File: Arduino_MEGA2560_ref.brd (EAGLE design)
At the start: 101.6 x 53.3 mm, 72 parts, among them IC1 MC33269ST-5.0T3, IC2 MC33269D-5.0, IC3 ATMEGA2560-16AU, IC4 ATMEGA8U2-MU, IC5 LM358D, IC6 LP2985-33DBVR, Q1 16MHz, Q2 16MHz, T2 FDN340P, X1 DC21MMX, Y1 16MHz, Y2 16MHz

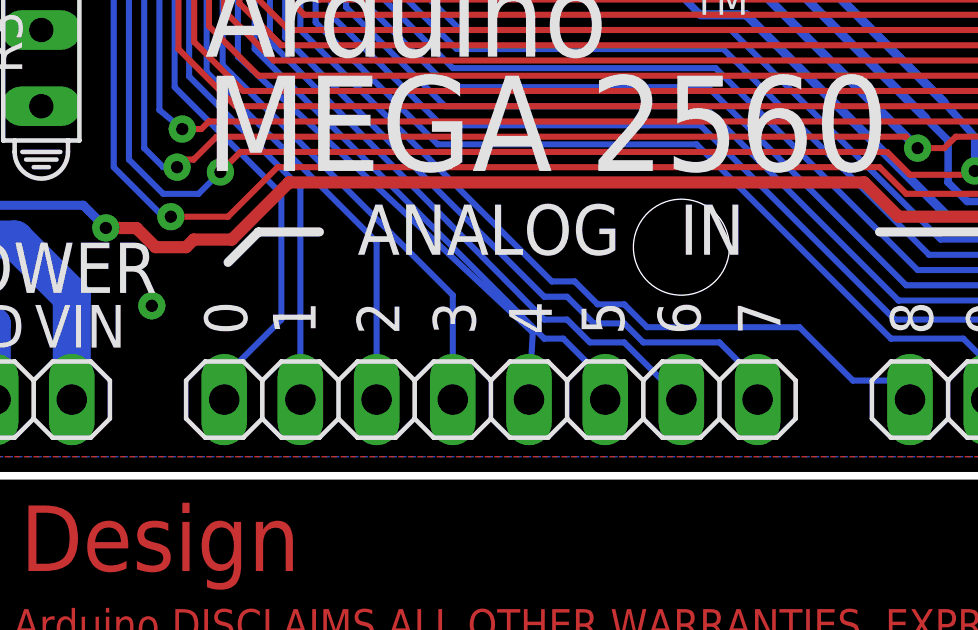
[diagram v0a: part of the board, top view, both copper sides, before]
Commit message: master changes
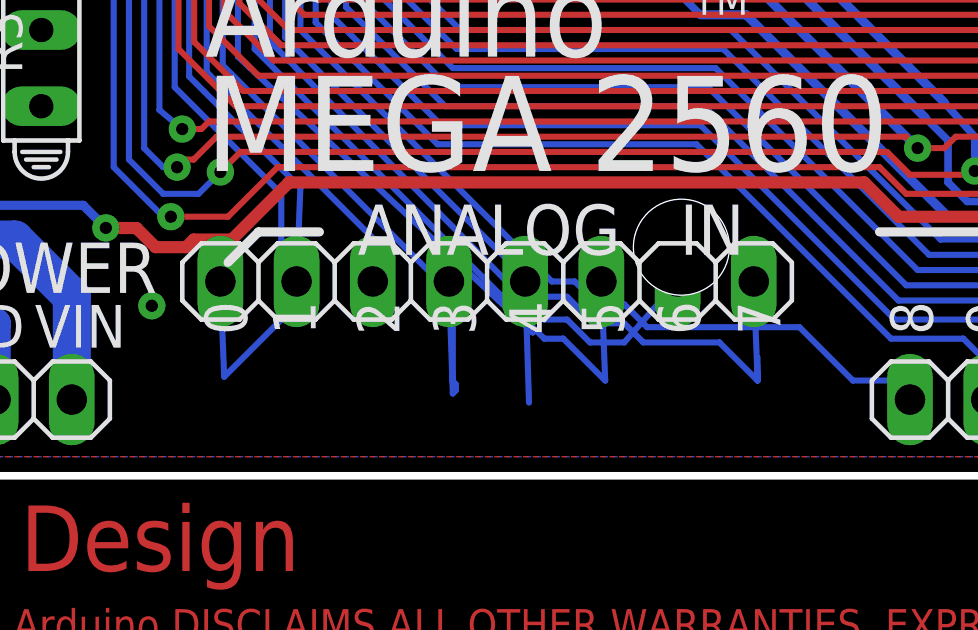
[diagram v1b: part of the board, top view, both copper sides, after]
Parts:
- moved ADCL 3.94 mm to (59.6, 6.48)
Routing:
- net ADC1: track 44.4 -> 40.5 mm
- net ADC2: track 46.9 -> 42.9 mm
- net ADC3: track 49.7 -> 53.3 mm
- net ADC4: track 52.9 -> 56.3 mm
- net ADC7: track 58.1 -> 60.8 mm
- net ADC5: track 55.9 -> 58.5 mm
- net ADC0: track 43.0 -> 45.4 mm
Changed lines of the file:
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@@
 <attribute name="VALUE" x="13.716" y="16.256" size="1.27" layer="27" rot="R90"/>
 </element>
-<element name="ADCL" library="pinhead" package="1X08" value="" x="59.69" y="2.54" smashed="yes">
-<attribute name="NAME" x="57.6326" y="4.7498" size="1.27" layer="49" ratio="10"/>
-<attribute name="VALUE" x="49.53" y="-0.635" size="1.27" layer="27"/>
+<element name="ADCL" library="pinhead" package="1X08" value="" x="59.563" y="6.477" smashed="yes">
+<attribute name="NAME" x="57.5056" y="8.6868" size="1.27" layer="49" ratio="10"/>
+<attribute name="VALUE" x="49.403" y="3.302" size="1.27" layer="27"/>
 </element>
 <element name="COMMUNICATION" library="pinhead" package="1X08" value="" x="77.47" y="50.8" smashed="yes" rot="R180">
@@
 <wire x1="52.705" y1="5.207" x2="52.705" y2="9.398" width="0.2032" layer="16"/>
 <wire x1="50.8" y1="3.302" x2="52.705" y2="5.207" width="0.2032" layer="16"/>
-<wire x1="50.8" y1="2.54" x2="50.8" y2="3.302" width="0.2032" layer="16"/>
+<wire x1="50.673" y1="6.477" x2="50.8" y2="3.302" width="0.2032" layer="16"/>
 <wire x1="46.3" y1="37.52" x2="46.3" y2="36.3464" width="0.2032" layer="1"/>
 <wire x1="46.228" y1="25.273" x2="46.228" y2="37.592" width="0.2032" layer="16"/>
@@
 <contactref element="ADCL" pad="3"/>
 <contactref element="IC3" pad="95"/>
-<wire x1="55.88" y1="2.54" x2="55.88" y2="7.7978" width="0.2032" layer="16"/>
+<wire x1="55.753" y1="6.477" x2="55.88" y2="7.7978" width="0.2032" layer="16"/>
 <wire x1="47.371" y1="36.576" x2="47.3" y2="36.505" width="0.2032" layer="1"/>
 <wire x1="47.2694" y1="36.6776" x2="47.371" y2="36.576" width="0.2032" layer="1"/>
@@
 <wire x1="49.6316" y1="13.3096" x2="49.6316" y2="22.5552" width="0.2032" layer="16"/>
 <wire x1="53.34" y1="9.6012" x2="49.6316" y2="13.3096" width="0.2032" layer="16"/>
-<wire x1="53.34" y1="2.54" x2="53.34" y2="9.6012" width="0.2032" layer="16"/>
+<wire x1="53.213" y1="6.477" x2="53.34" y2="9.6012" width="0.2032" layer="16"/>
 <wire x1="46.8" y1="37.655" x2="46.8" y2="36.3464" width="0.2032" layer="1"/>
 <wire x1="46.482" y1="37.973" x2="46.8" y2="37.655" width="0.2032" layer="1"/>
@@
 <wire x1="58.42" y1="3.1496" x2="58.42" y2="6.0198" width="0.2032" layer="16"/>
 <wire x1="58.5216" y1="3.048" x2="58.42" y2="3.1496" width="0.2032" layer="16"/>
-<wire x1="58.42" y1="2.54" x2="58.42" y2="2.7432" width="0.2032" layer="16"/>
+<wire x1="58.293" y1="6.477" x2="58.42" y2="2.7432" width="0.2032" layer="16"/>
 <wire x1="58.5216" y1="2.8448" x2="58.5216" y2="3.048" width="0.2032" layer="16"/>
 <wire x1="58.42" y1="2.7432" x2="58.5216" y2="2.8448" width="0.2032" layer="16"/>
@@
 <wire x1="51.2572" y1="13.97" x2="51.2572" y2="23.0632" width="0.2032" layer="16"/>
 <wire x1="61.087" y1="4.7752" x2="51.2572" y2="13.97" width="0.2032" layer="16"/>
-<wire x1="60.96" y1="2.4384" x2="60.96" y2="2.54" width="0.2032" layer="16"/>
-<wire x1="60.96" y1="2.54" x2="61.087" y2="4.7752" width="0.2032" layer="16"/>
+<wire x1="60.96" y1="2.4384" x2="60.833" y2="6.477" width="0.2032" layer="16"/>
+<wire x1="60.833" y1="6.477" x2="61.087" y2="4.7752" width="0.2032" layer="16"/>
 <wire x1="48.3" y1="38.06" x2="48.3" y2="36.3464" width="0.2032" layer="1"/>
 <wire x1="48.006" y1="38.354" x2="48.3" y2="38.06" width="0.2032" layer="1"/>
@@
 <wire x1="62.103" y1="4.572" x2="61.468" y2="4.572" width="0.2032" layer="16"/>
 <wire x1="62.103" y1="4.572" x2="63.5" y2="3.175" width="0.2032" layer="16"/>
-<wire x1="63.5" y1="3.175" x2="63.5" y2="2.54" width="0.2032" layer="16"/>
+<wire x1="63.5" y1="3.175" x2="63.373" y2="6.477" width="0.2032" layer="16"/>
 <via x="49.657" y="43.561" extent="1-16" drill="0.4064" shape="octagon"/>
 </signal>
@@
 <wire x1="62.992" y1="4.445" x2="62.23" y2="5.207" width="0.2032" layer="16"/>
 <wire x1="62.992" y1="4.445" x2="64.135" y2="4.445" width="0.2032" layer="16"/>
-<wire x1="64.135" y1="4.445" x2="66.04" y2="2.54" width="0.2032" layer="16"/>
+<wire x1="64.135" y1="4.445" x2="65.913" y2="6.477" width="0.2032" layer="16"/>
 <via x="49.276" y="39.37" extent="1-16" drill="0.4064" shape="octagon"/>
 </signal>
@@
 <wire x1="52.832" y1="14.605" x2="52.832" y2="23.368" width="0.2032" layer="16"/>
 <wire x1="52.832" y1="14.605" x2="61.468" y2="5.969" width="0.2032" layer="16"/>
-<wire x1="68.58" y1="3.175" x2="68.58" y2="2.54" width="0.2032" layer="16"/>
+<wire x1="68.58" y1="3.175" x2="68.453" y2="6.477" width="0.2032" layer="16"/>
 <wire x1="68.58" y1="3.175" x2="68.58" y2="3.937" width="0.2032" layer="16"/>
 <wire x1="64.77" y1="4.445" x2="67.31" y2="4.445" width="0.2032" layer="16"/>

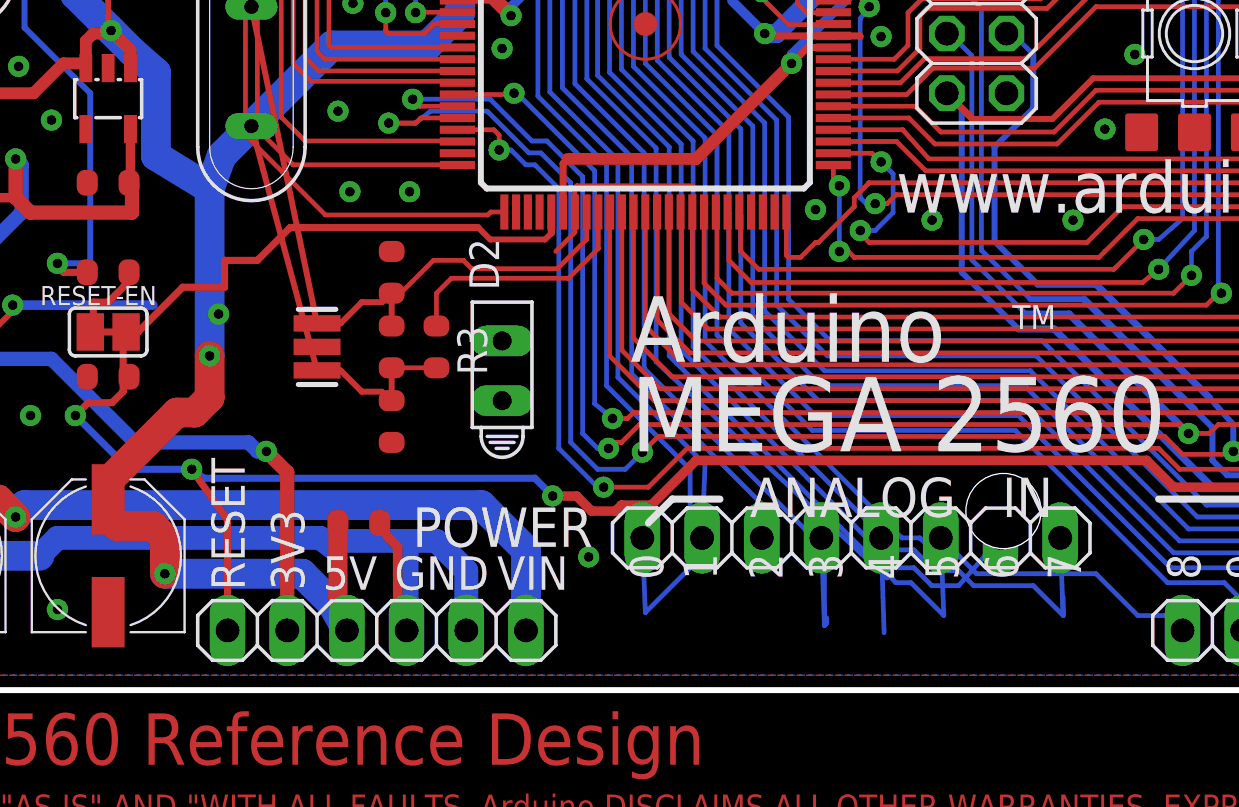
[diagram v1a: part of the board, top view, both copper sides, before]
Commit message: feature branch created with some changes
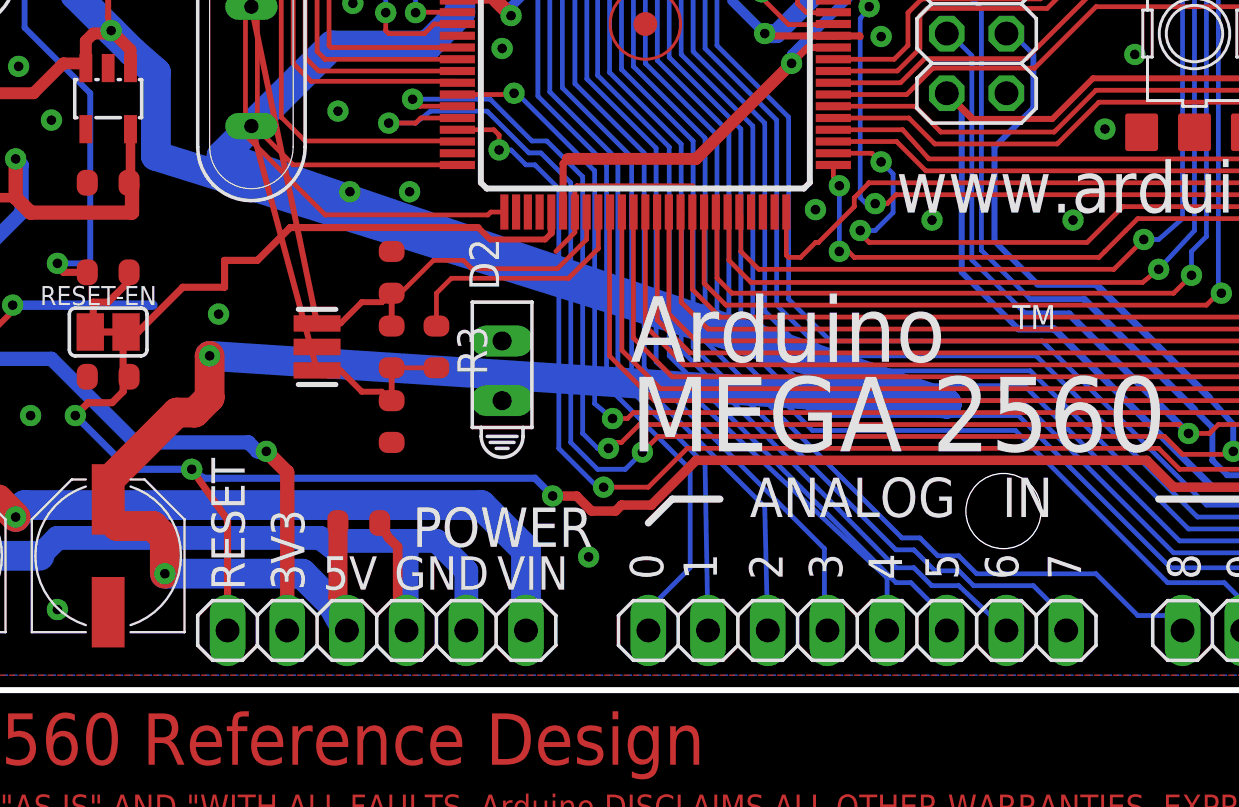
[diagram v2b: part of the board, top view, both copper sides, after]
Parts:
- moved ADCL 3.95 mm to (59.8, 2.54)
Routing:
- net +5V: track 291.7 -> 379.7 mm
- net ADC1: track 40.5 -> 44.4 mm
- net ADC2: track 42.9 -> 46.9 mm
- net ADC3: track 53.3 -> 49.8 mm
- net ADC4: track 56.3 -> 53.0 mm
- net ADC7: track 60.8 -> 58.1 mm
- net ADC5: track 58.5 -> 55.9 mm
- net ADC0: track 45.4 -> 43.0 mm
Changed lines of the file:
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@@
 <attribute name="VALUE" x="13.716" y="16.256" size="1.27" layer="27" rot="R90"/>
 </element>
-<element name="ADCL" library="pinhead" package="1X08" value="" x="59.563" y="6.477" smashed="yes">
-<attribute name="NAME" x="57.5056" y="8.6868" size="1.27" layer="49" ratio="10"/>
-<attribute name="VALUE" x="49.403" y="3.302" size="1.27" layer="27"/>
+<element name="ADCL" library="pinhead" package="1X08" value="" x="59.817" y="2.54" smashed="yes">
+<attribute name="NAME" x="57.7596" y="4.7498" size="1.27" layer="49" ratio="10"/>
+<attribute name="VALUE" x="49.657" y="-0.635" size="1.27" layer="27"/>
 </element>
 <element name="COMMUNICATION" library="pinhead" package="1X08" value="" x="77.47" y="50.8" smashed="yes" rot="R180">
@@
 <wire x1="18.796" y1="34.544" x2="18.038" y2="35.302" width="0.3048" layer="1"/>
 <wire x1="29.972" y1="22.733" x2="29.972" y2="26.289" width="1.27" layer="16"/>
-<wire x1="32.258" y1="21.336" x2="29.972" y2="22.733" width="1.27" layer="16"/>
-<wire x1="32.258" y1="14.224" x2="32.258" y2="21.336" width="1.27" layer="16"/>
+<wire x1="63.627" y1="12.192" x2="29.972" y2="22.733" width="1.27" layer="16"/>
+<wire x1="32.258" y1="14.224" x2="63.627" y2="12.192" width="1.27" layer="16"/>
 <wire x1="32.258" y1="14.224" x2="32.258" y2="14.986" width="0" layer="19" extent="1-16"/>
 <wire x1="37.465" y1="27.432" x2="41.529" y2="27.432" width="1.27" layer="16"/>
 <wire x1="32.766" y1="22.733" x2="37.465" y2="27.432" width="1.27" layer="16"/>
-<wire x1="32.258" y1="21.336" x2="32.766" y2="22.733" width="1.27" layer="16"/>
+<wire x1="63.627" y1="12.192" x2="32.766" y2="22.733" width="1.27" layer="16"/>
 <wire x1="29.972" y1="26.289" x2="28.956" y2="27.178" width="1.27" layer="16"/>
 <wire x1="28.956" y1="27.178" x2="28.067" y2="28.067" width="1.27" layer="16"/>
@@
 <wire x1="52.705" y1="5.207" x2="52.705" y2="9.398" width="0.2032" layer="16"/>
 <wire x1="50.8" y1="3.302" x2="52.705" y2="5.207" width="0.2032" layer="16"/>
-<wire x1="50.673" y1="6.477" x2="50.8" y2="3.302" width="0.2032" layer="16"/>
+<wire x1="50.927" y1="2.54" x2="50.8" y2="3.302" width="0.2032" layer="16"/>
 <wire x1="46.3" y1="37.52" x2="46.3" y2="36.3464" width="0.2032" layer="1"/>
 <wire x1="46.228" y1="25.273" x2="46.228" y2="37.592" width="0.2032" layer="16"/>
@@
 <contactref element="ADCL" pad="3"/>
 <contactref element="IC3" pad="95"/>
-<wire x1="55.753" y1="6.477" x2="55.88" y2="7.7978" width="0.2032" layer="16"/>
+<wire x1="56.007" y1="2.54" x2="55.88" y2="7.7978" width="0.2032" layer="16"/>
 <wire x1="47.371" y1="36.576" x2="47.3" y2="36.505" width="0.2032" layer="1"/>
 <wire x1="47.2694" y1="36.6776" x2="47.371" y2="36.576" width="0.2032" layer="1"/>
@@
 <wire x1="49.6316" y1="13.3096" x2="49.6316" y2="22.5552" width="0.2032" layer="16"/>
 <wire x1="53.34" y1="9.6012" x2="49.6316" y2="13.3096" width="0.2032" layer="16"/>
-<wire x1="53.213" y1="6.477" x2="53.34" y2="9.6012" width="0.2032" layer="16"/>
+<wire x1="53.467" y1="2.54" x2="53.34" y2="9.6012" width="0.2032" layer="16"/>
 <wire x1="46.8" y1="37.655" x2="46.8" y2="36.3464" width="0.2032" layer="1"/>
 <wire x1="46.482" y1="37.973" x2="46.8" y2="37.655" width="0.2032" layer="1"/>
@@
 <wire x1="58.42" y1="3.1496" x2="58.42" y2="6.0198" width="0.2032" layer="16"/>
 <wire x1="58.5216" y1="3.048" x2="58.42" y2="3.1496" width="0.2032" layer="16"/>
-<wire x1="58.293" y1="6.477" x2="58.42" y2="2.7432" width="0.2032" layer="16"/>
+<wire x1="58.547" y1="2.54" x2="58.42" y2="2.7432" width="0.2032" layer="16"/>
 <wire x1="58.5216" y1="2.8448" x2="58.5216" y2="3.048" width="0.2032" layer="16"/>
 <wire x1="58.42" y1="2.7432" x2="58.5216" y2="2.8448" width="0.2032" layer="16"/>
@@
 <wire x1="51.2572" y1="13.97" x2="51.2572" y2="23.0632" width="0.2032" layer="16"/>
 <wire x1="61.087" y1="4.7752" x2="51.2572" y2="13.97" width="0.2032" layer="16"/>
-<wire x1="60.96" y1="2.4384" x2="60.833" y2="6.477" width="0.2032" layer="16"/>
-<wire x1="60.833" y1="6.477" x2="61.087" y2="4.7752" width="0.2032" layer="16"/>
+<wire x1="60.96" y1="2.4384" x2="61.087" y2="2.54" width="0.2032" layer="16"/>
+<wire x1="61.087" y1="2.54" x2="61.087" y2="4.7752" width="0.2032" layer="16"/>
 <wire x1="48.3" y1="38.06" x2="48.3" y2="36.3464" width="0.2032" layer="1"/>
 <wire x1="48.006" y1="38.354" x2="48.3" y2="38.06" width="0.2032" layer="1"/>
@@
 <wire x1="62.103" y1="4.572" x2="61.468" y2="4.572" width="0.2032" layer="16"/>
 <wire x1="62.103" y1="4.572" x2="63.5" y2="3.175" width="0.2032" layer="16"/>
-<wire x1="63.5" y1="3.175" x2="63.373" y2="6.477" width="0.2032" layer="16"/>
+<wire x1="63.5" y1="3.175" x2="63.627" y2="2.54" width="0.2032" layer="16"/>
 <via x="49.657" y="43.561" extent="1-16" drill="0.4064" shape="octagon"/>
 </signal>
@@
 <wire x1="62.992" y1="4.445" x2="62.23" y2="5.207" width="0.2032" layer="16"/>
 <wire x1="62.992" y1="4.445" x2="64.135" y2="4.445" width="0.2032" layer="16"/>
-<wire x1="64.135" y1="4.445" x2="65.913" y2="6.477" width="0.2032" layer="16"/>
+<wire x1="64.135" y1="4.445" x2="66.167" y2="2.54" width="0.2032" layer="16"/>
 <via x="49.276" y="39.37" extent="1-16" drill="0.4064" shape="octagon"/>
 </signal>
@@
 <wire x1="52.832" y1="14.605" x2="52.832" y2="23.368" width="0.2032" layer="16"/>
 <wire x1="52.832" y1="14.605" x2="61.468" y2="5.969" width="0.2032" layer="16"/>
-<wire x1="68.58" y1="3.175" x2="68.453" y2="6.477" width="0.2032" layer="16"/>
+<wire x1="68.58" y1="3.175" x2="68.707" y2="2.54" width="0.2032" layer="16"/>
 <wire x1="68.58" y1="3.175" x2="68.58" y2="3.937" width="0.2032" layer="16"/>
 <wire x1="64.77" y1="4.445" x2="67.31" y2="4.445" width="0.2032" layer="16"/>
